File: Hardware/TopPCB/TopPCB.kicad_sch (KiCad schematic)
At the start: 5 parts

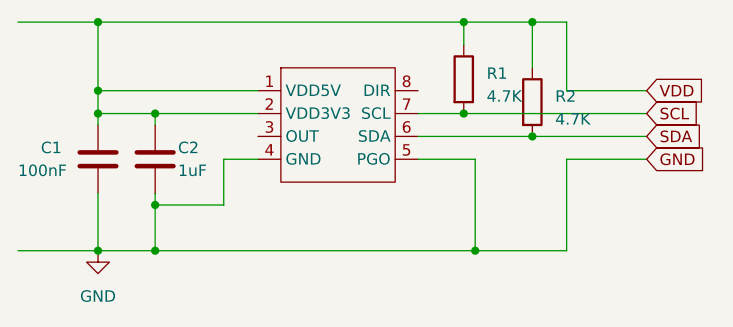
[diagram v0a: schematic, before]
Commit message: updated ibom
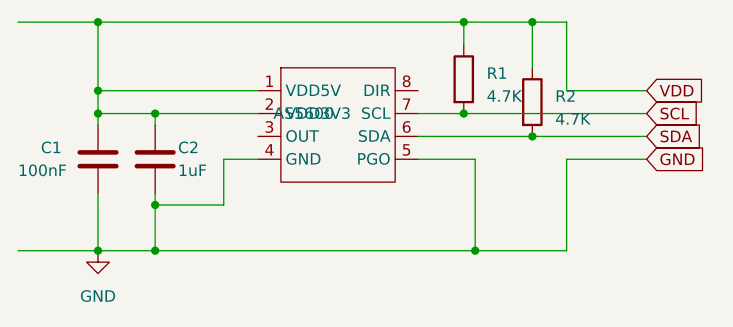
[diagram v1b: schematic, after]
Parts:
- U1: value ~ -> AS5600
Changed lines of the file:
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@@
       (effects (font (size 1.27 1.27)) hide)
     )
-    (property "Value" "~" (at 109.22 85.09 0)
+    (property "Value" "AS5600" (at 109.22 85.09 0)
       (effects (font (size 1.27 1.27)))
     )
